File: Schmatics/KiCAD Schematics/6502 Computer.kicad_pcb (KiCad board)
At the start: 2 copper layers, 188.3 x 114.3 mm, 51 parts, among them J10 Conn_02x01, J11 RCJ-017, J12 Conn_02x03_Odd_Even, J13 Conn_02x01, J2 Conn_02x20_Odd_Even, J3 Conn_01x04_Male, J4 Conn_02x03_Odd_Even, J5 Conn_02x08_Odd_Even, J6 Conn_01x06_Male, J7 Conn_02x03_Odd_Even, J8 Barrel_Jack, J9 Conn_01x11_Male, P1 Mini-DIN_6pins, SW1 RESET, U1 WD65C02, U2 28C256, U3 WC1602A, U4 74HC00, U5 WD65C22, U6 CY62256-70PC, U7 6551, U8 74HC166, U9 LM7805_TO220, X1 ACO-1.8432MHz, Y1 11.0582 MHz, Y2 16 MHz

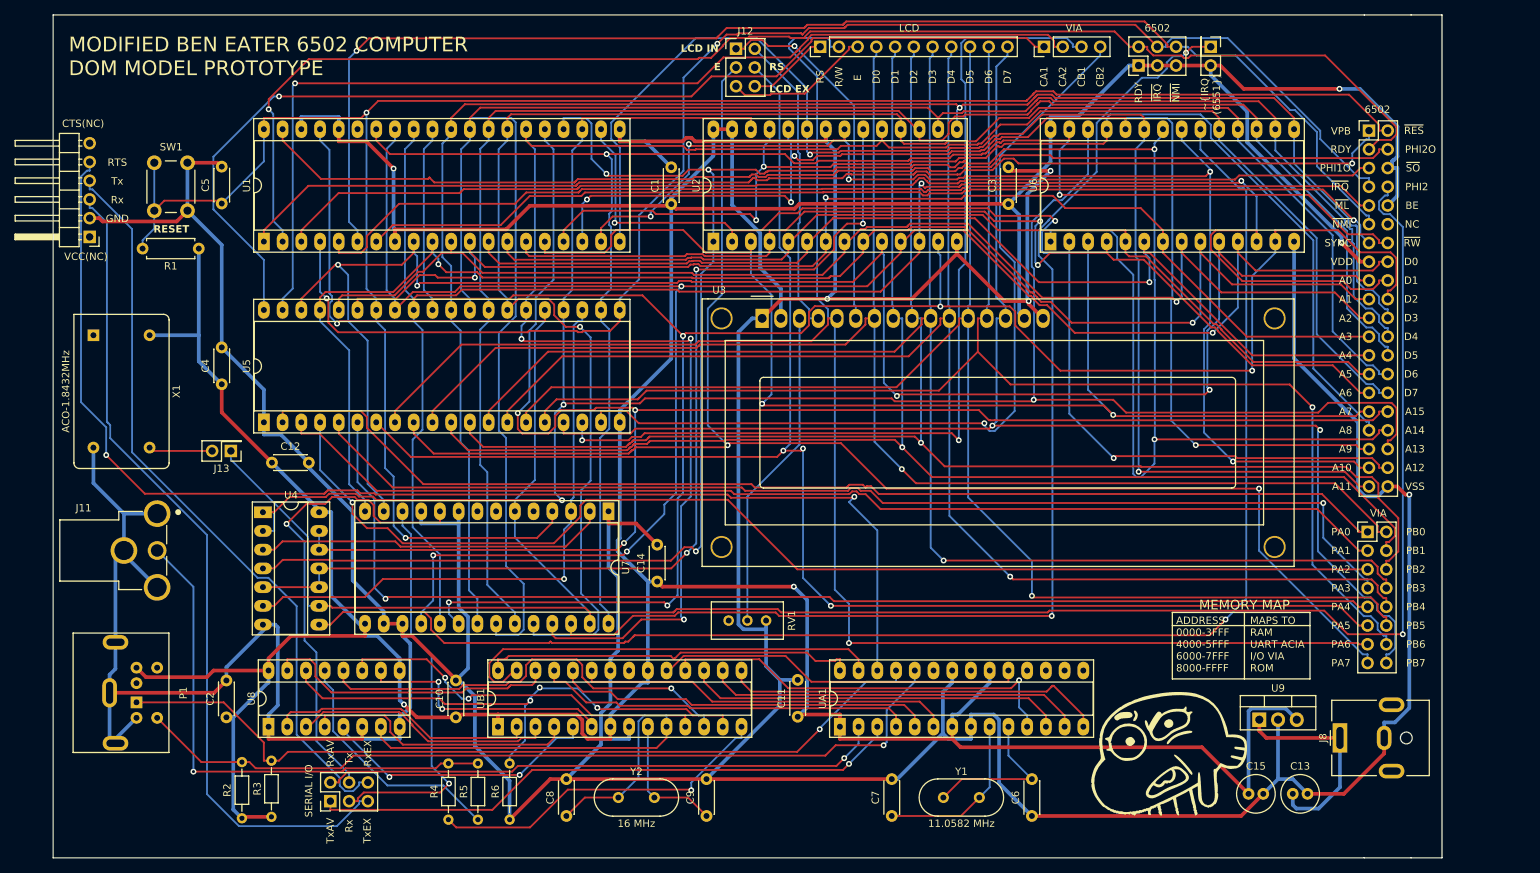
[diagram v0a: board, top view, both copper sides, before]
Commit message: MAJOR push with big basic improvements
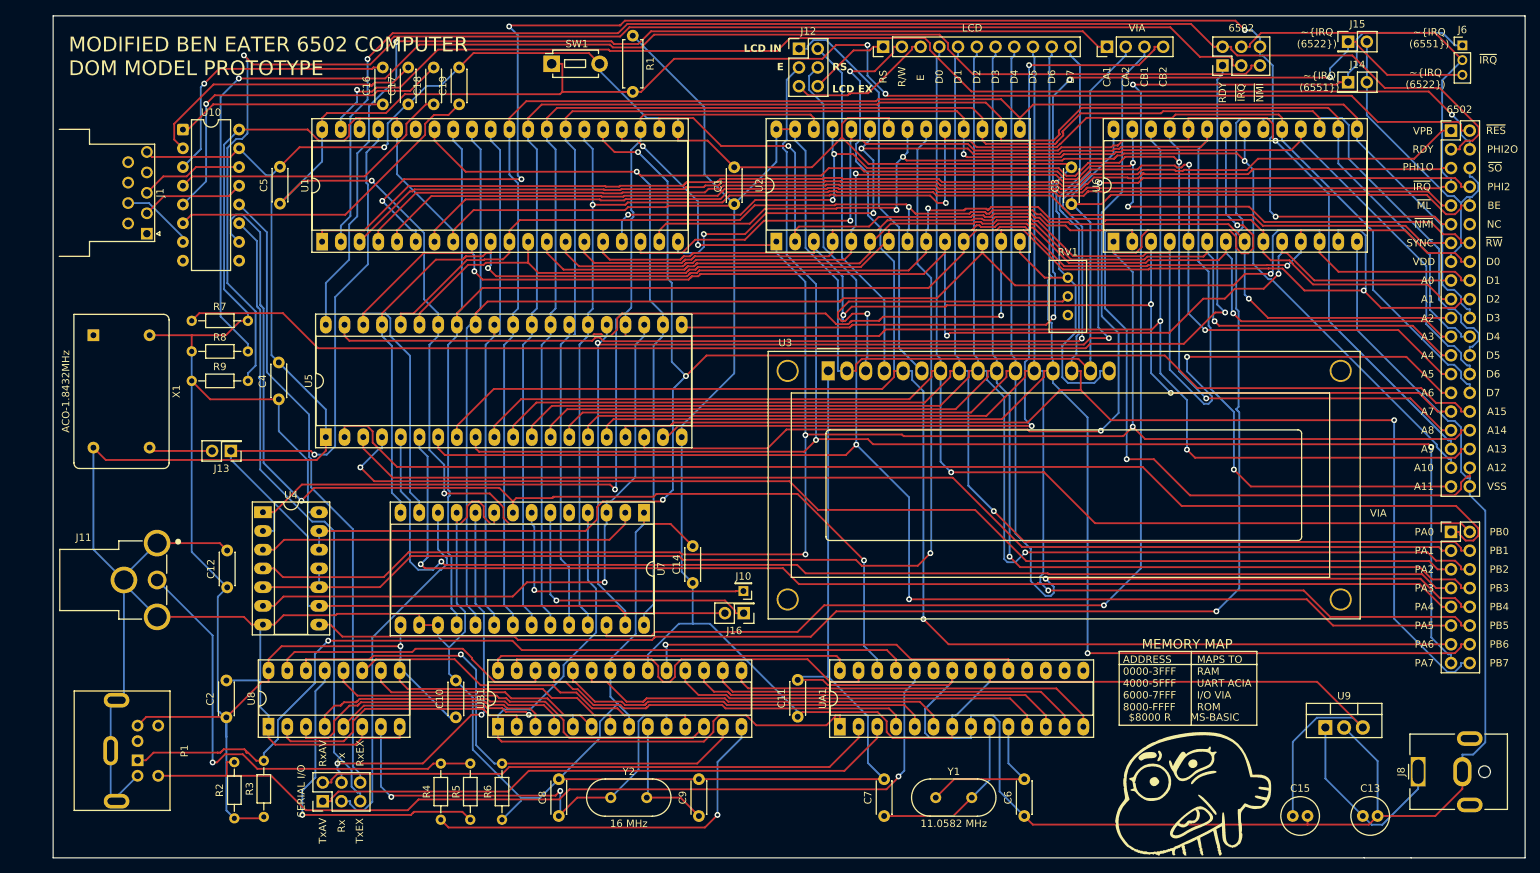
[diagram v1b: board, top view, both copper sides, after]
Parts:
- added C16: 1uf, Capacitor_THT:C_Disc_D4.3mm_W1.9mm_P5.00mm, F.Cu at (70.1, 28.0)
- added C17: 1uf, Capacitor_THT:C_Disc_D4.3mm_W1.9mm_P5.00mm, F.Cu at (73.5, 28.0)
- added C18: 1uf, Capacitor_THT:C_Disc_D4.3mm_W1.9mm_P5.00mm, F.Cu at (77.0, 28.0)
- added C19: 1uf, Capacitor_THT:C_Disc_D4.3mm_W1.9mm_P5.00mm, F.Cu at (80.5, 28.0)
- added J1: DE9_Pins, Connector_Dsub:DSUB-9_Socket_Horizontal_P2.77x2.54mm_EdgePinOffset9.40mm, F.Cu at (38.1, 45.5)
- added J14: Conn_02x01, Connector_PinHeader_2.54mm:PinHeader_2x01_P2.54mm_Vertical, F.Cu at (201.0, 25.0)
- added J15: Conn_02x01, Connector_PinHeader_2.54mm:PinHeader_2x01_P2.54mm_Vertical, F.Cu at (201.0, 19.5)
- added J16: Conn_02x01, Connector_PinHeader_2.54mm:PinHeader_2x01_P2.54mm_Vertical, F.Cu at (119.0, 97.0)
- added R7: 10k, Resistor_THT:R_Axial_DIN0204_L3.6mm_D1.6mm_P7.62mm_Horizontal, F.Cu at (44.2, 57.4)
- added R8: 10k, Resistor_THT:R_Axial_DIN0204_L3.6mm_D1.6mm_P7.62mm_Horizontal, F.Cu at (44.2, 61.5)
- added R9: 10k, Resistor_THT:R_Axial_DIN0204_L3.6mm_D1.6mm_P7.62mm_Horizontal, F.Cu at (44.2, 65.5)
- added U10: MAX232, Package_DIP:DIP-16_W7.62mm, F.Cu at (43.0, 31.4)
- J10: value Conn_02x01 -> Conn_01x01; footprint Connector_PinHeader_2.54mm:PinHeader_2x01_P2.54mm_Vertical -> Connector_PinHeader_2.00mm:PinHeader_1x01_P2.00mm_Vertical
- J6: value Conn_01x06_Male -> Conn_01x03; footprint Connector_PinHeader_2.54mm:PinHeader_1x06_P2.54mm_Horizontal -> Connector_PinHeader_2.00mm:PinHeader_1x03_P2.00mm_Vertical
- SW1: footprint Button_Switch_THT:SW_PUSH_6mm_H5mm -> Button_Switch_THT:SW_PUSH_1P1T_6x3.5mm_H4.3_APEM_MJTP1243
- moved J6 188.0 mm to (216.5, 20.0), turned to 0 degrees
- moved J10 97.3 mm to (119.0, 94.0), turned to 180 degrees
- moved R1 65.6 mm to (104.0, 18.7), turned to -90 degrees
- moved RV1 61.9 mm to (163.0, 51.5), turned to 0 degrees
- moved SW1 57.4 mm to (93.0, 22.5), turned to 0 degrees
- moved C12 18.0 mm to (49.0, 93.5), turned to 90 degrees
- moved J8 11.5 mm to (210.5, 118.5)
- moved U3 11.4 mm to (130.5, 64.1)
- moved J7 11.4 mm to (184.0, 22.7)
- moved J5 11.3 mm to (215.0, 86.0)
- moved J2 11.1 mm to (215.0, 31.6)
- moved C13 9.96 mm to (203.0, 124.5)
- moved U9 9.02 mm to (197.9, 112.5)
- moved U5 8.64 mm to (62.4, 73.1)
- moved J3 8.54 mm to (168.3, 20.2)
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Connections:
- J6 pad 1: unconnected-(J6-Pin_1-Pad1) -> Net-(J14-Pin_1)
- J6 pad 2: GND -> Net-(J2-Pin_7)
- J6 pad 3: Net-(J4-Pin_5) -> Net-(J15-Pin_1)
- J7 pad 1: +5V -> Net-(J7-Pin_1)
- J7 pad 3: +5V -> Net-(J7-Pin_3)
- J7 pad 5: +5V -> Net-(J7-Pin_5)
- U5 pad 21: Net-(J2-Pin_7) -> Net-(J15-Pin_1)
- U7 pad 26: Net-(J10-Pin_1) -> Net-(J14-Pin_1)
- U7 pad 6: Net-(J13-Pin_1) -> Net-(J16-Pin_1)
- U7 pad 7: unconnected-(U7-XLT0-Pad7) -> Net-(J10-Pin_1)
- U7 pad 8: unconnected-(U7-~{RTS}-Pad8) -> Net-(U10-T2IN)
- UA1 pad 1: +5V -> Net-(J2-Pin_2)
- UA1 pad 26: Net-(J6-Pin_5) -> Net-(U10-T2IN)
- UB1 pad 1: +5V -> Net-(J2-Pin_2)
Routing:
- net Net-(J14-Pin_1): track 0.00 -> 194.8 mm, vias 0 -> 2
- net Net-(J7-Pin_3): track 0.00 -> 188.7 mm, vias 0 -> 1
- net Net-(J7-Pin_5): track 0.00 -> 184.2 mm, vias 0 -> 1
- net Net-(J7-Pin_1): track 0.00 -> 179.0 mm, vias 0 -> 1
- net Net-(J6-Pin_5): track 171.9 -> 0.00 mm, vias 2 -> 0
- net Net-(U10-T2IN): track 0.00 -> 147.1 mm, vias 0 -> 2
- net Net-(J15-Pin_1): track 0.00 -> 143.5 mm, vias 0 -> 3
- net Net-(J10-Pin_1): track 159.3 -> 39.1 mm, vias 2 -> 1
- net +5V: track 689.5 -> 781.9 mm, vias 5 -> 1
- net Net-(J2-Pin_2): track 275.2 -> 361.7 mm, vias 2 -> 4
- net GND: track 814.1 -> 896.2 mm, vias 4 -> 1
- net Net-(U10-C2-): track 0.00 -> 47.8 mm, vias 0 -> 1
- net Net-(U10-VS-): track 0.00 -> 45.0 mm
- net Net-(U10-C2+): track 0.00 -> 39.4 mm
- net Net-(U10-VS+): track 0.00 -> 39.1 mm
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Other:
- board size 188.3 x 114.3 mm -> 199.6 x 114.2 mm
- board text added: "$8000 R MS-BASIC"
- board text added: "~{IRQ (6522})"
- board text removed: "CTS(NC)"
- board text removed: "GND"
- board text removed: "RESET"
- board text removed: "RTS"
- board text removed: "VCC(NC)"
